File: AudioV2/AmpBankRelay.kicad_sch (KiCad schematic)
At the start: 17 parts, among them K301 AZ850P2-5, K302 AZ850P2-5, K303 AZ850P2-5, K304 AZ850P2-5, U321 TBD62083APG

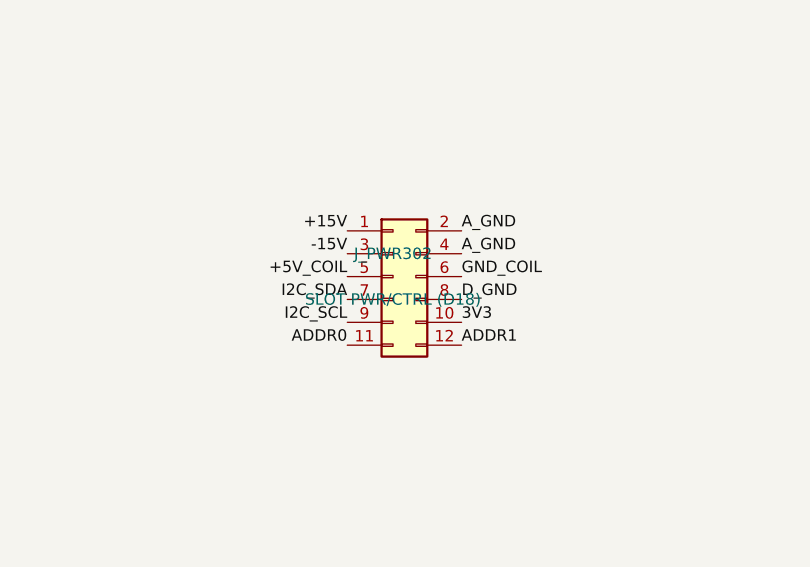
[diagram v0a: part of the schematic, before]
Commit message: re asighn pin
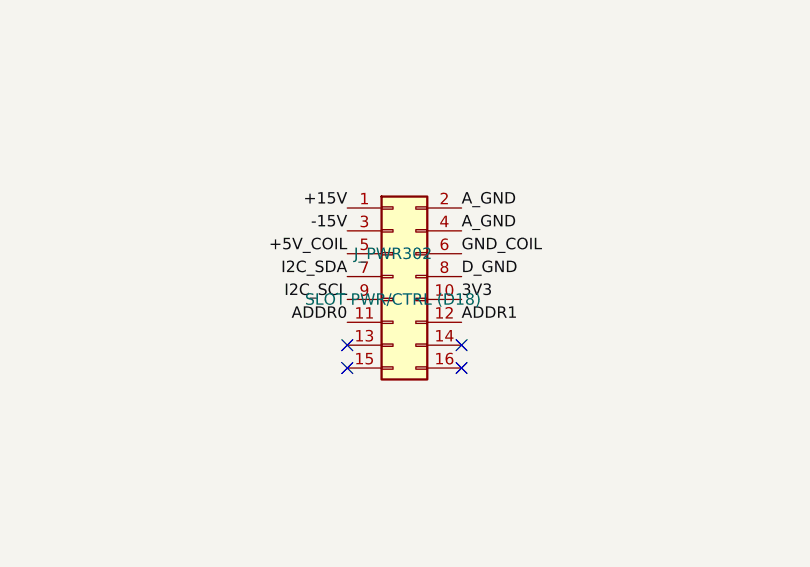
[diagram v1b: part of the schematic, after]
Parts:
- removed H311: M3, MountingHole:MountingHole_3.2mm_M3, symbol Mechanical:MountingHole
- removed J_PWR302: SLOT PWR/CTRL (D18), Connector_PinHeader_2.54mm:PinHeader_2x06_P2.54mm_Vertical, symbol Connector_Generic:Conn_02x06_Odd_Even
- added C322: 100nF, Capacitor_SMD:C_1206_3216Metric_Pad1.33x1.80mm_HandSolder, symbol Device:C
- added J_PWR302: SLOT PWR/CTRL (D18), Connector_PinHeader_2.54mm:PinHeader_2x08_P2.54mm_Vertical, symbol Connector_Generic:Conn_02x08_Odd_Even
- H311: renamed from C322; value 100nF -> M3; footprint Capacitor_SMD:C_1206_3216Metric_Pad1.33x1.80mm_HandSolder -> MountingHole:MountingHole_3.2mm_M3; symbol Device:C -> Mechanical:MountingHole
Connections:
- net +15V: now also J_PWR302.1 (Pin_1)
- net +5V_COIL: now also C322.1, J_PWR302.5 (Pin_5); no longer H311.1
- net -15V: now also J_PWR302.3 (Pin_3)
- net 3V3: now also J_PWR302.10 (Pin_10)
- net ADDR0: now also J_PWR302.11 (Pin_11)
- net ADDR1: now also J_PWR302.12 (Pin_12)
- net A_GND: now also J_PWR302.2 (Pin_2), J_PWR302.4 (Pin_4)
- net D_GND: now also J_PWR302.8 (Pin_8)
- net GND_COIL: now also C322.2, J_PWR302.6 (Pin_6); no longer H311.2
- net I2C_SCL: now also J_PWR302.9 (Pin_9)
- net I2C_SDA: now also J_PWR302.7 (Pin_7)
- no-connect marks 20 -> 24
